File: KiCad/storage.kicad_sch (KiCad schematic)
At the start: 3 parts, among them IC11 KLMCG4JETD-B041, J5 Micro_SD_Card

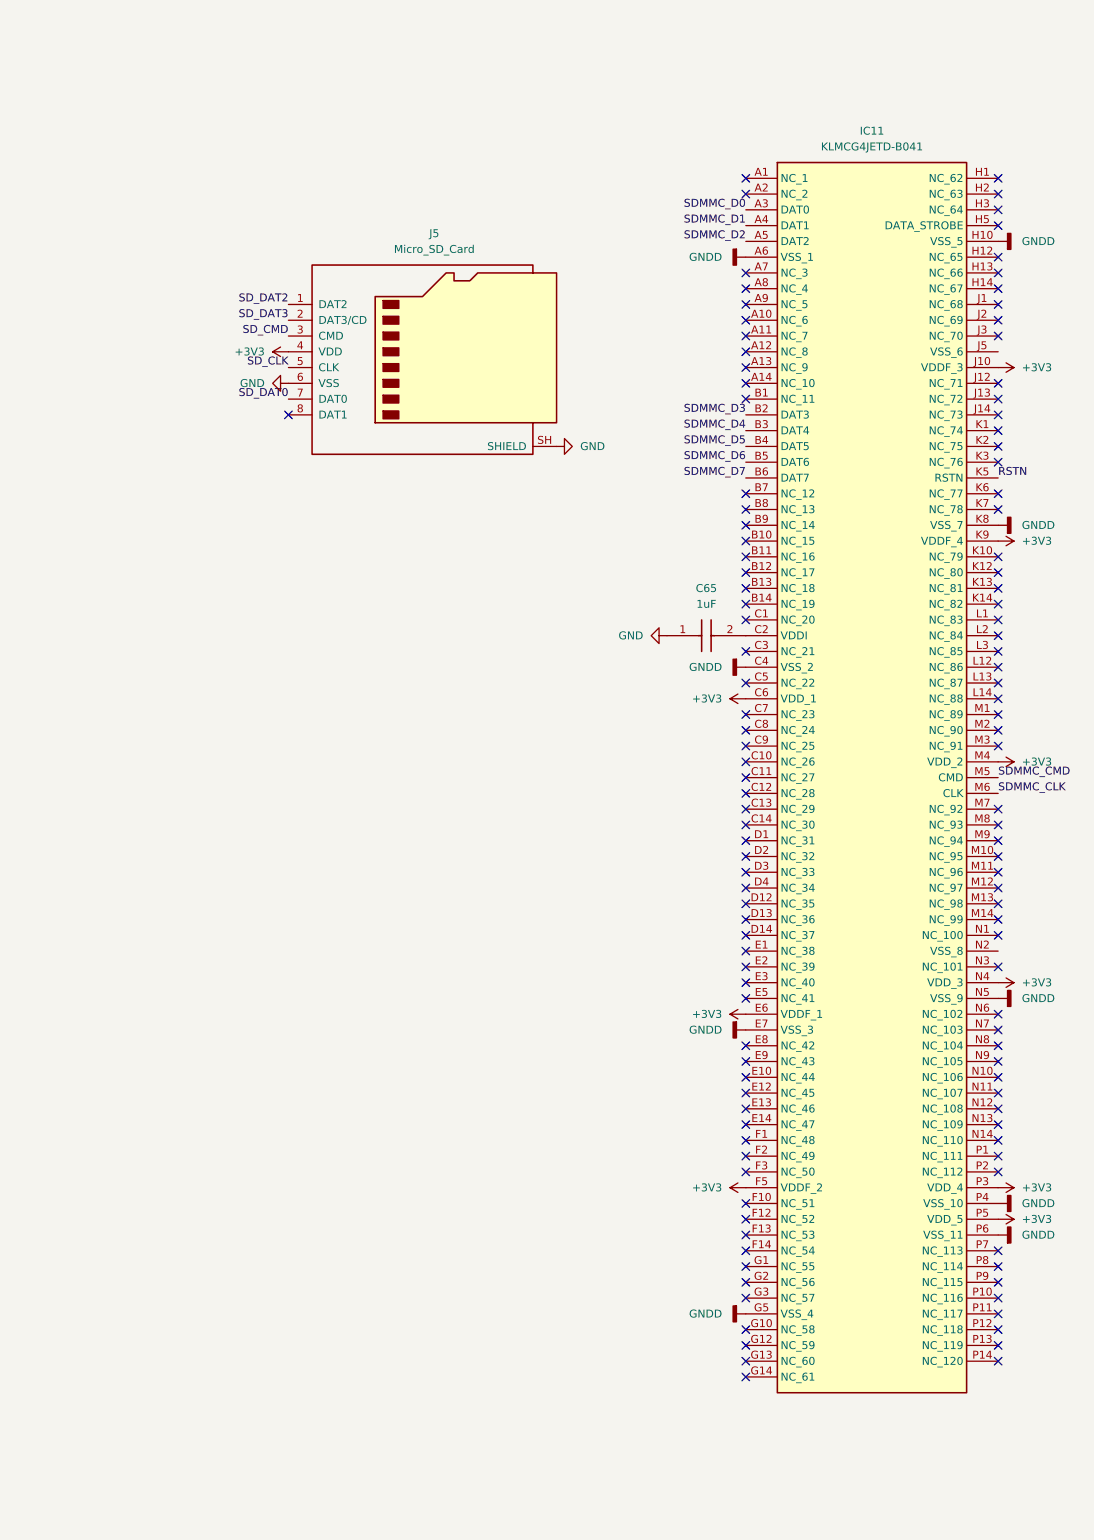
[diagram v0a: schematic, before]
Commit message: redesign
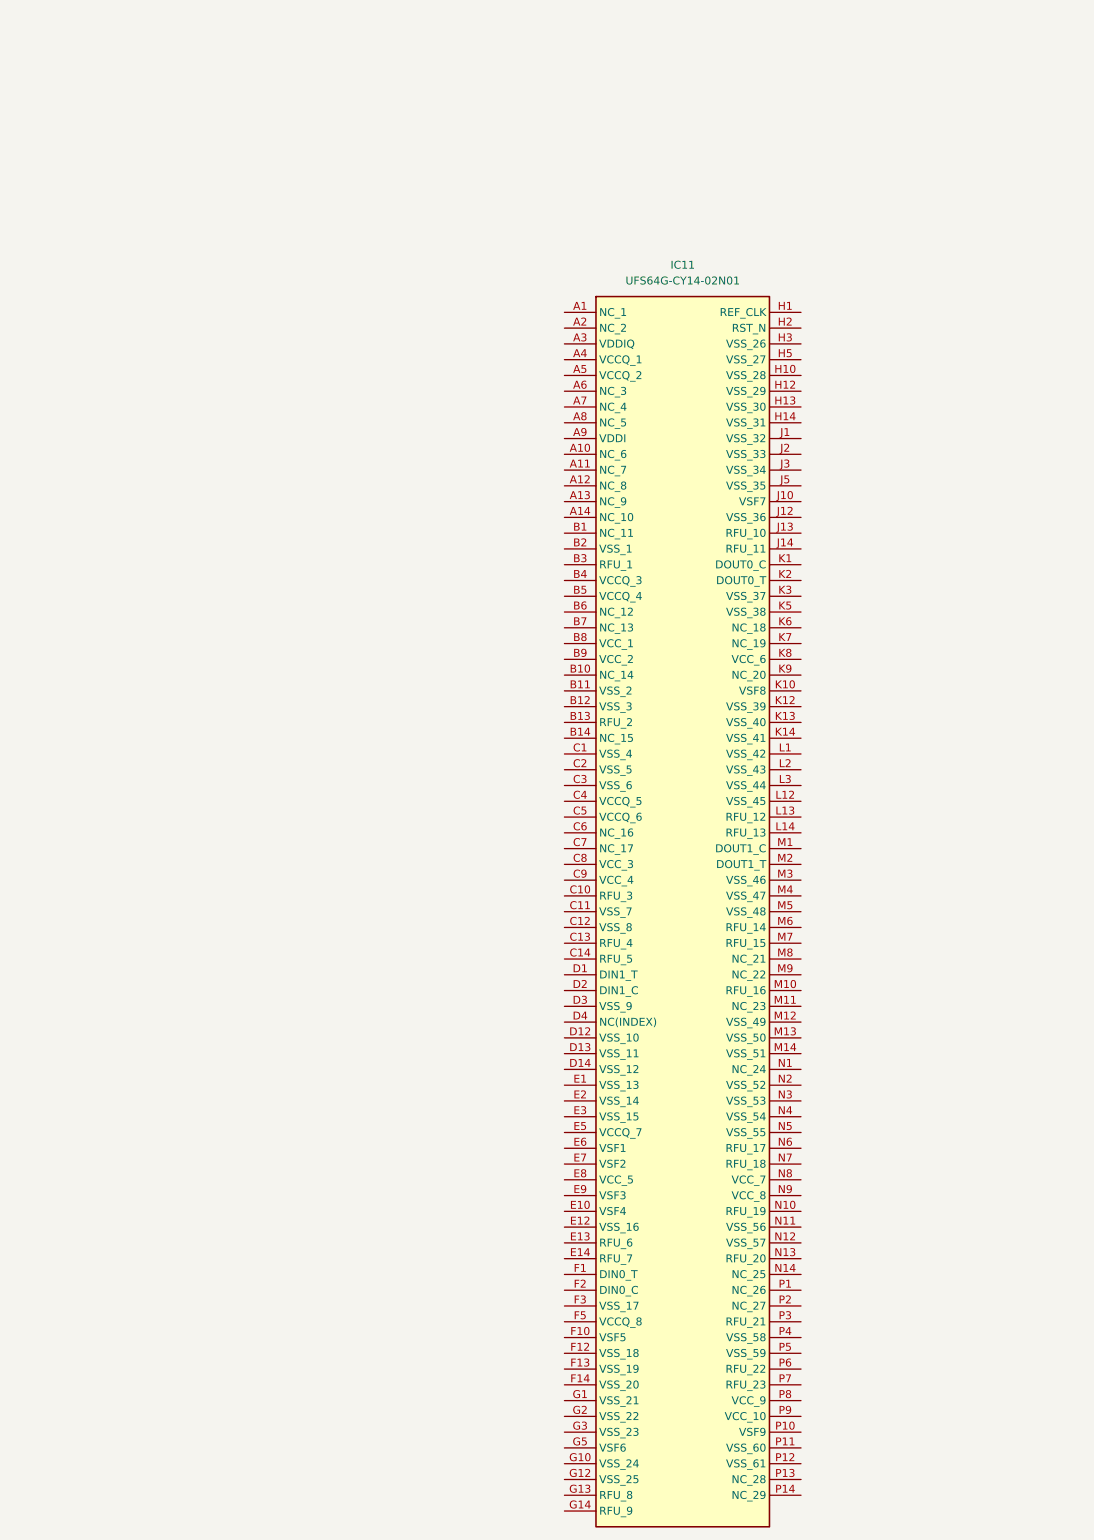
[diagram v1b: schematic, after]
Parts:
- removed C65: 1uF, Footprints:GRM155R61H334ME01D, symbol Symbols:GRM155D71E105KE11J
- removed IC11: KLMCG4JETD-B041, Footprints:BGA153C50P14X14_1150X1300X80, symbol Symbols:KLMAG1JETD-B041
- removed J5: Micro_SD_Card, Connector_Card:microSD_HC_Wuerth_693072010801, symbol Connector:Micro_SD_Card
- added IC11: UFS64G-CY14-02N01, BGA153C50P14X14_1100X1300X85, symbol Symbols:UFS64G-CY14-02N01
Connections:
- no-connect marks 122 -> 0

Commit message: aaaa
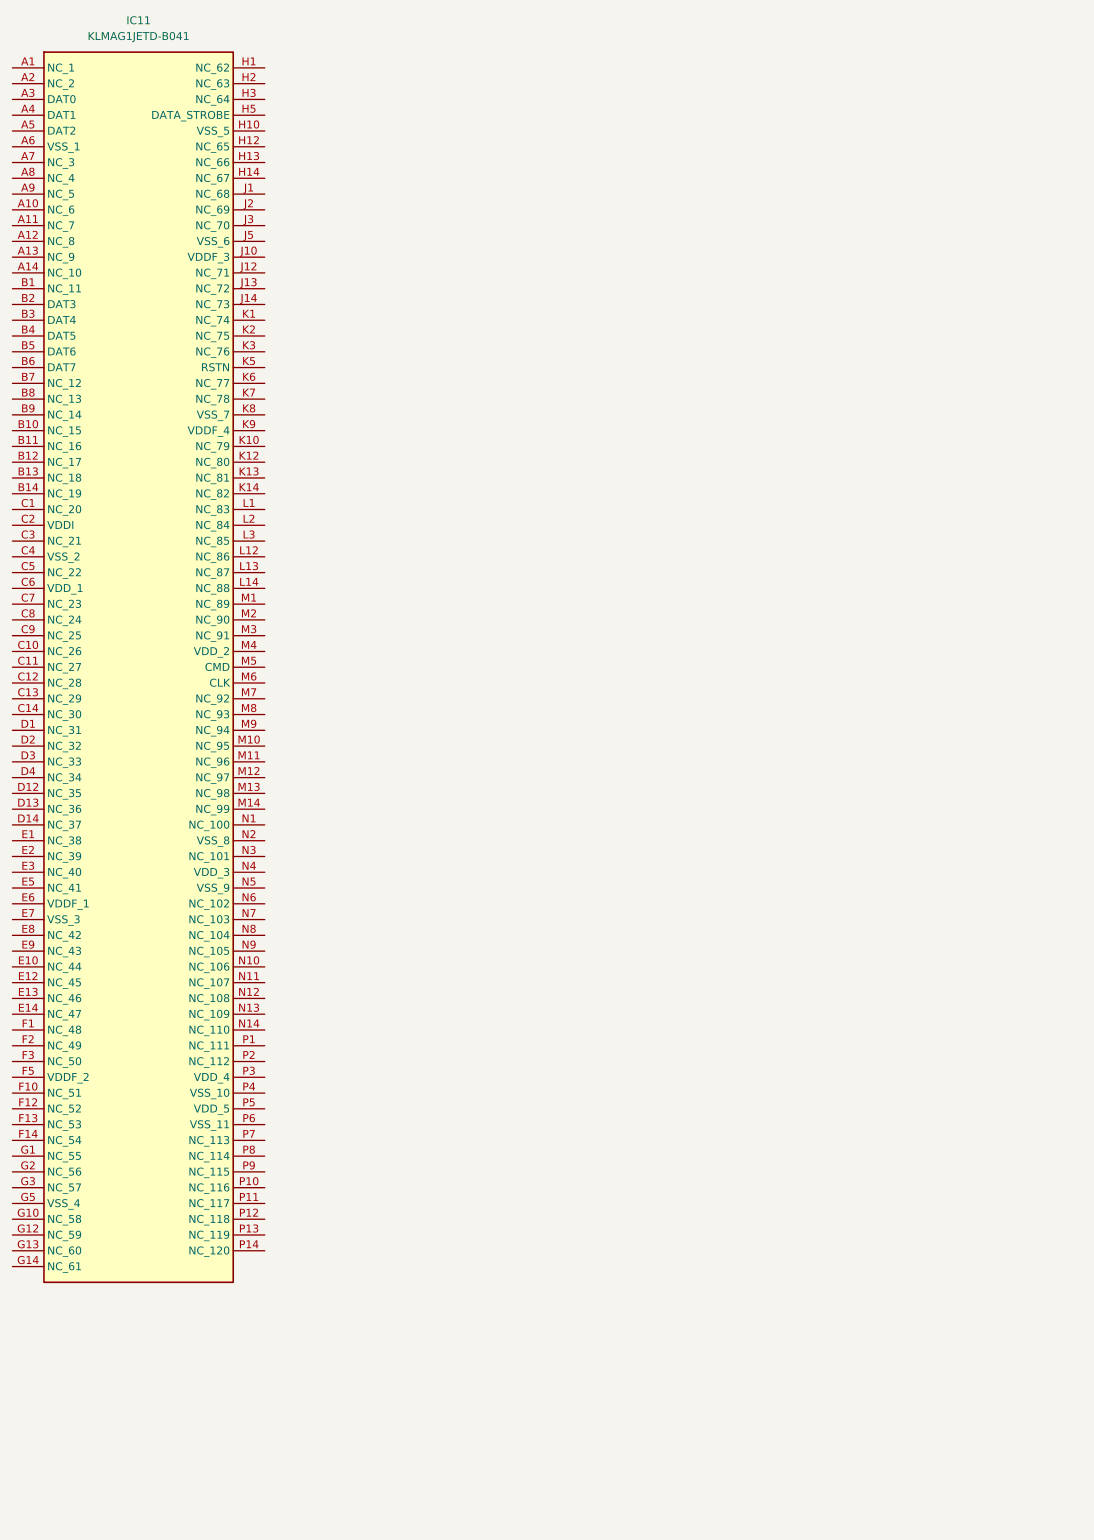
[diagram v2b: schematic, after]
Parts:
- removed IC11: UFS64G-CY14-02N01, BGA153C50P14X14_1100X1300X85, symbol Symbols:UFS64G-CY14-02N01
- added IC11: KLMAG1JETD-B041, BGA153C50P14X14_1150X1300X80, symbol Symbols:KLMAG1JETD-B041
